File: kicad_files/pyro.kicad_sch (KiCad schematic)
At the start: 14 parts, among them J12 IGN_1, J13 IGN_2, Q1 AO3400A, Q2 AO3400A

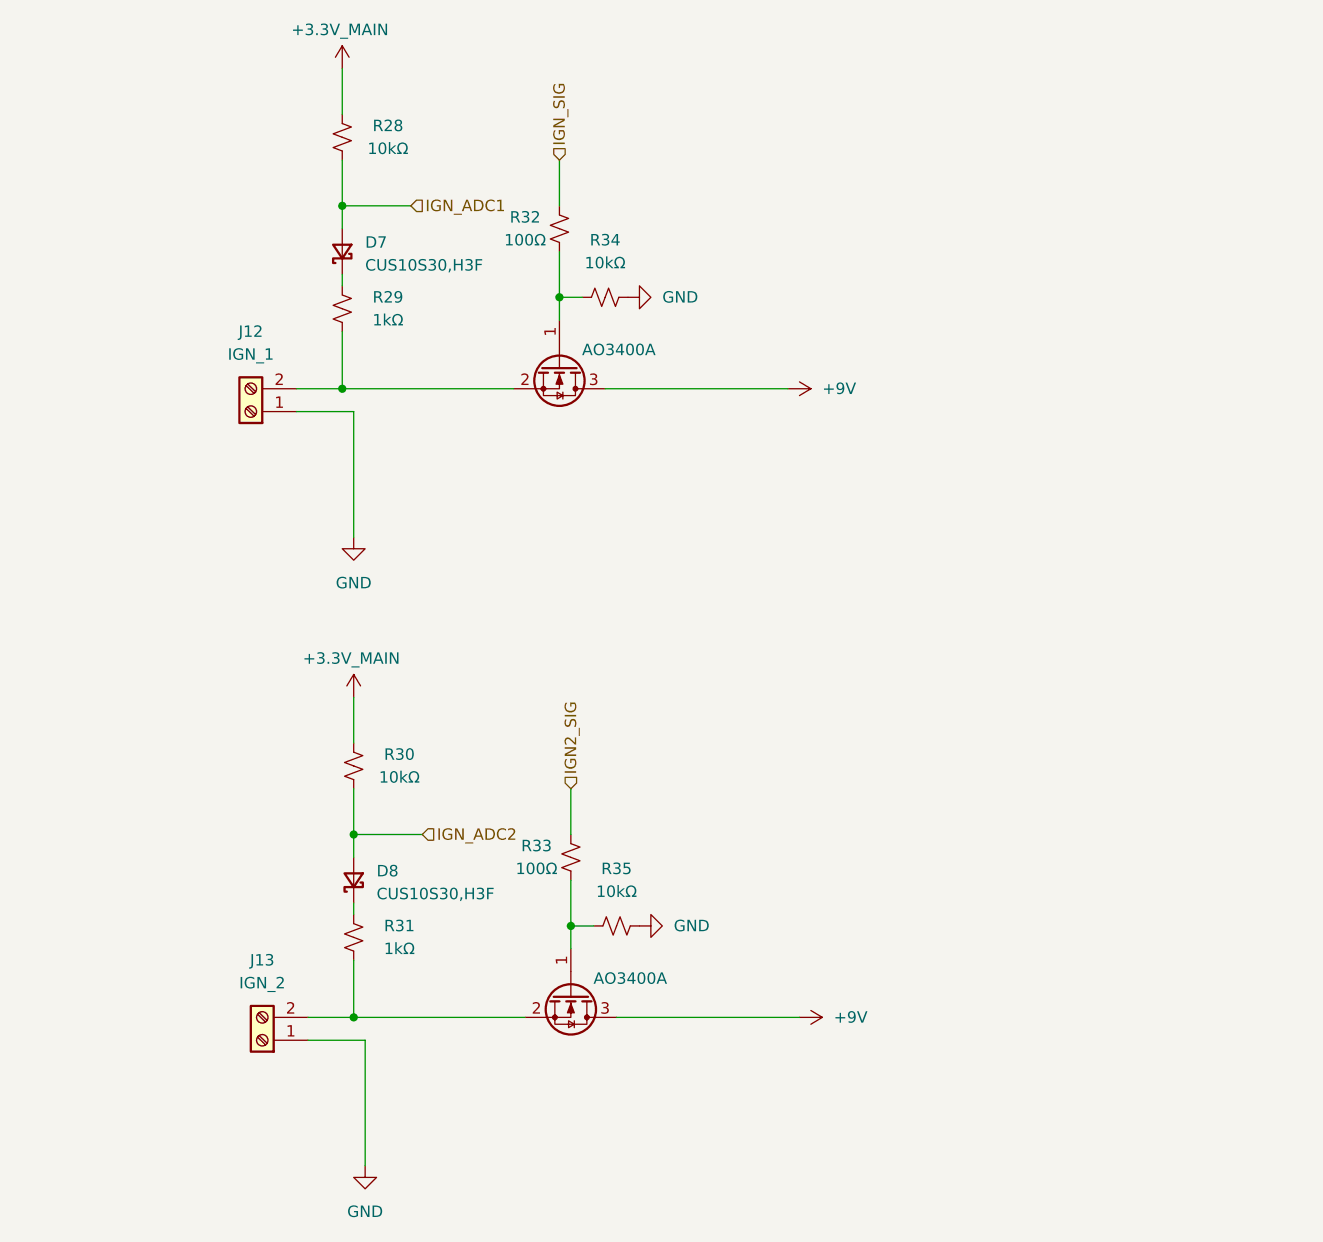
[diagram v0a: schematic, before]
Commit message: fix ign
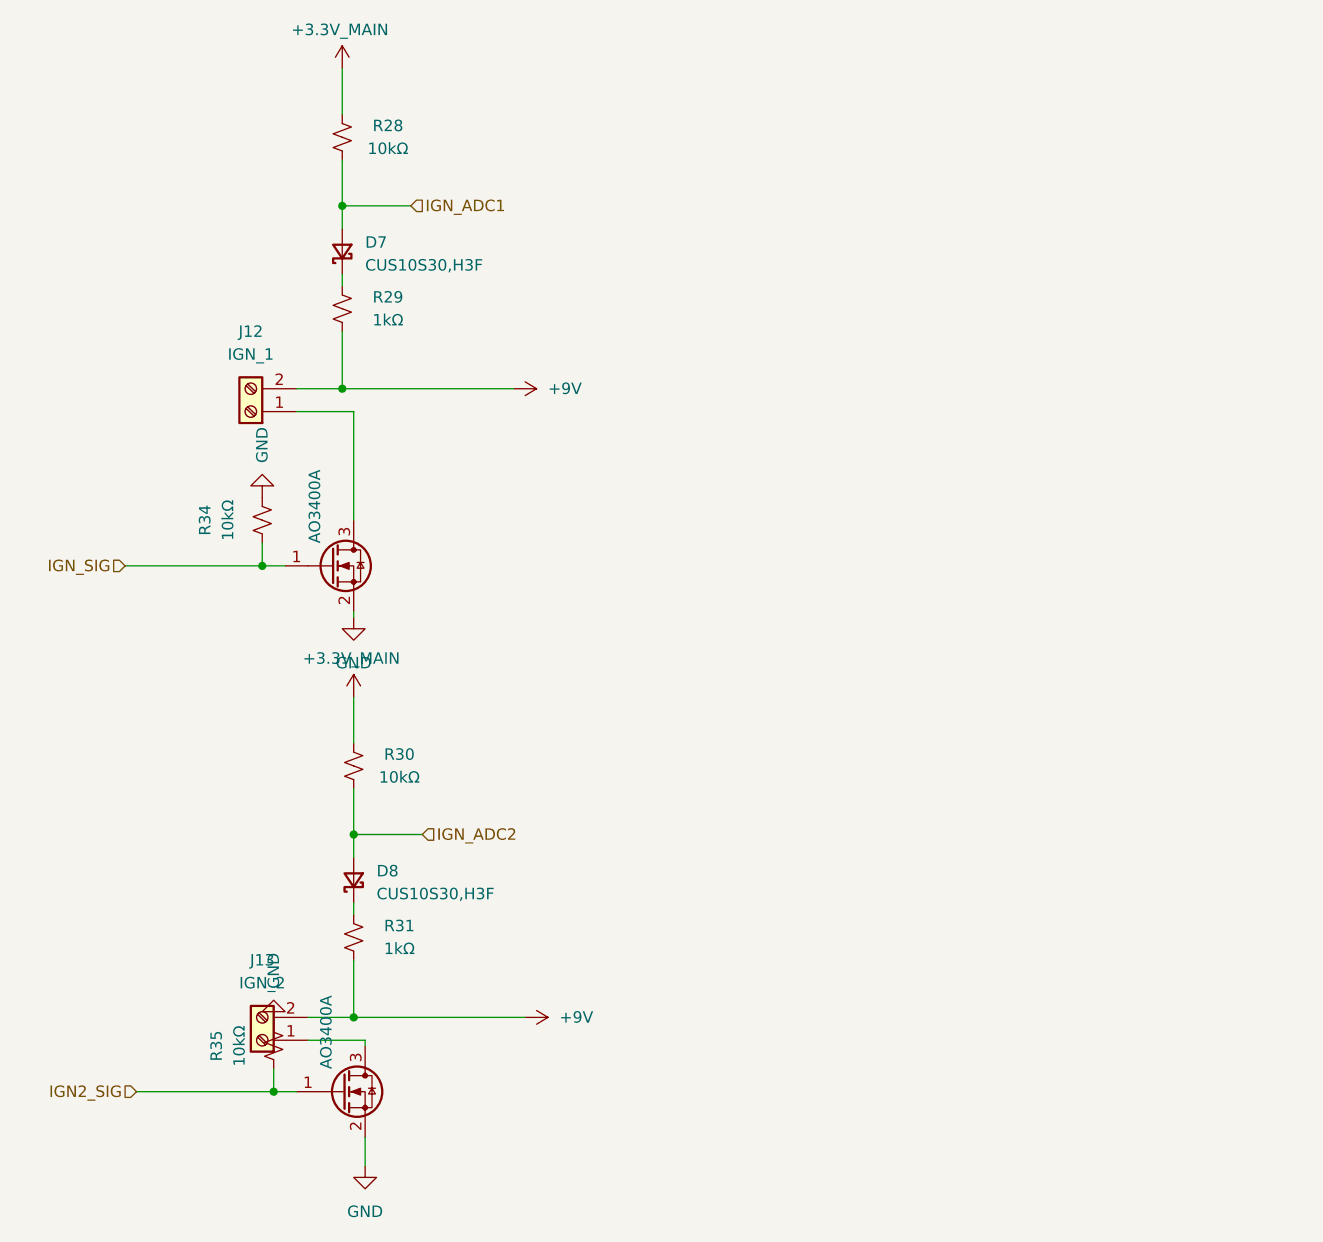
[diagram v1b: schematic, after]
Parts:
- removed R32, R33: 100Ω, Resistor_SMD:R_0603_1608Metric, symbol Device:R_Small_US
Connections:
- net +9V: now also J12.2 (Pin_2), J13.2 (Pin_2), R29.2, R31.2; no longer Q1.3 (D), Q2.3 (D)
- net GND: now also Q1.2 (S), Q2.2 (S); no longer J12.1 (Pin_1), J13.1 (Pin_1)
- net IGN2_SIG: now also Q2.1 (G), R35.1
- net IGN_SIG: now also Q1.1 (G), R34.1
- new net: J13.1 (Pin_1), Q2.3 (D)
- new net: J12.1 (Pin_1), Q1.3 (D)
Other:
- moved on the sheet: R34, R35

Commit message: fix pyro adc
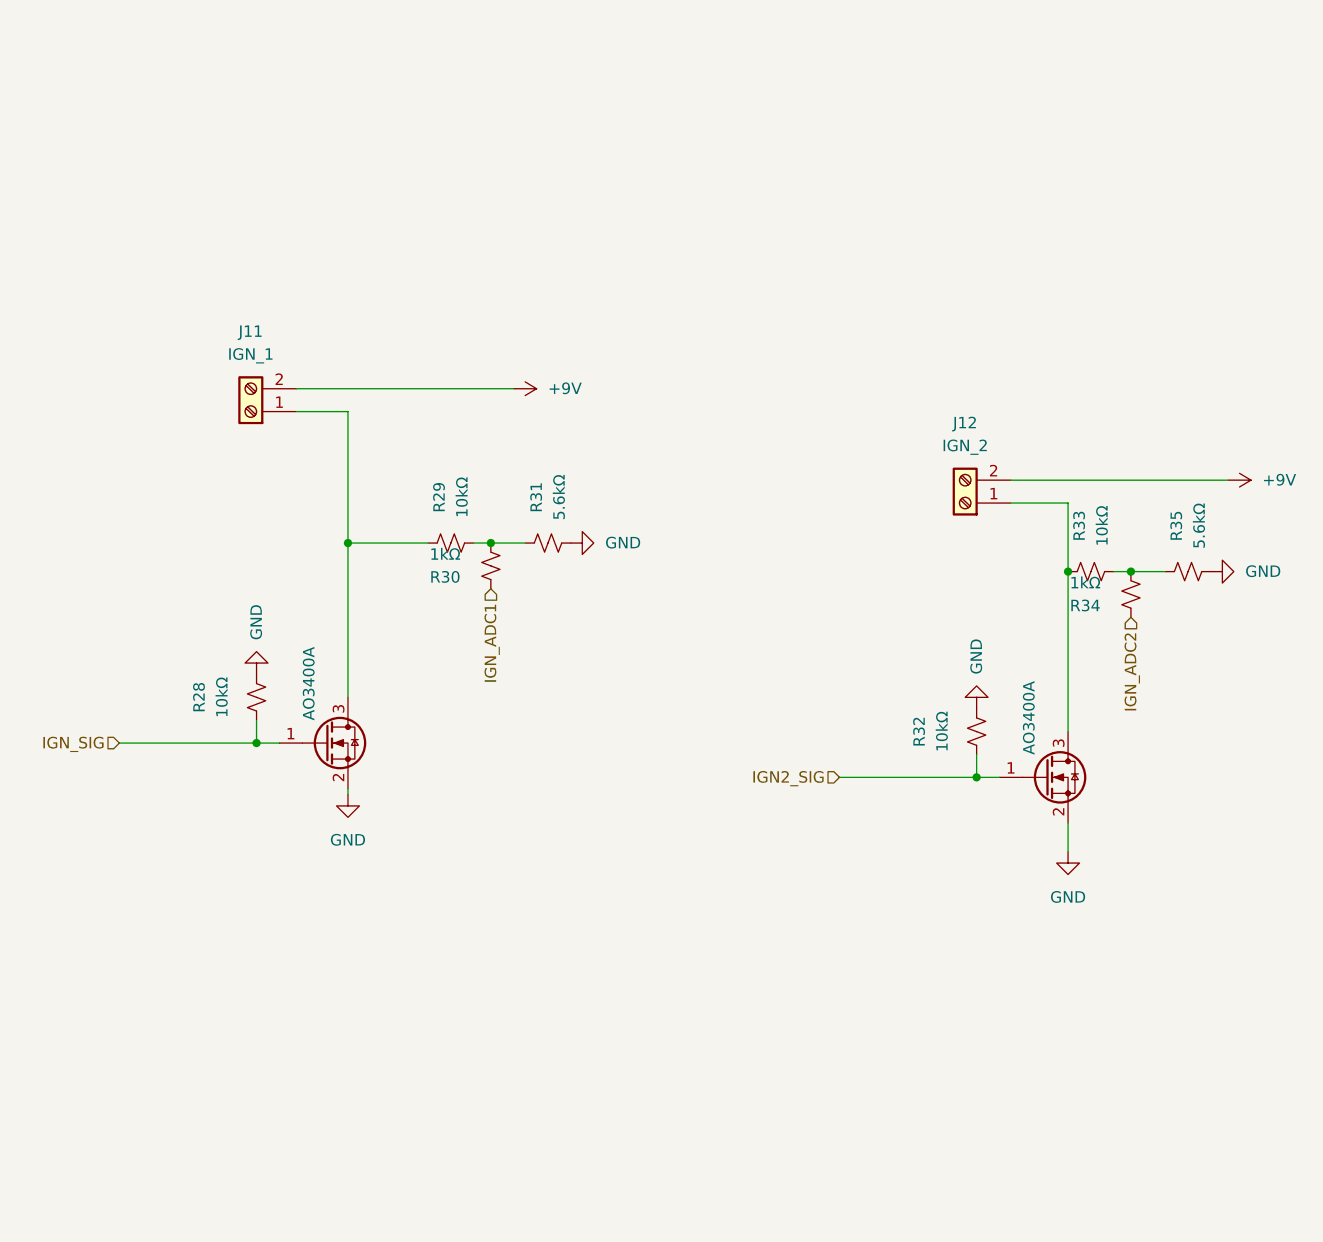
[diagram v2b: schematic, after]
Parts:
- removed D7, D8: CUS10S30,H3F, Diode_SMD:D_SOD-323, symbol Device:D_Schottky_Small
- removed R30: 10kΩ, Resistor_SMD:R_0402_1005Metric, symbol Device:R_Small_US
- added R33: 10kΩ, Resistor_SMD:R_0402_1005Metric, symbol Device:R_Small_US
- added R34: 1kΩ, Resistor_SMD:R_0402_1005Metric, symbol Device:R_Small_US
- added R35: 5.6kΩ, Resistor_SMD:R_0402_1005Metric, symbol Device:R_Small_US
- R30: renamed from R29; footprint Resistor_SMD:R_0805_2012Metric -> Resistor_SMD:R_0402_1005Metric
- R31: value 1kΩ -> 5.6kΩ; footprint Resistor_SMD:R_0805_2012Metric -> Resistor_SMD:R_0402_1005Metric
- renumbered J12 to J11, J13 to J12, R34 to R28, R28 to R29, R35 to R32
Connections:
- net +3.3V_MAIN is gone; now on an unnamed net: R29.1
- net +9V: no longer R30.2, R31.2
- net GND: now also R31.2, R35.2
- net IGN_ADC1: now also R30.1; no longer R29.2
- net IGN_ADC2: now also R34.1
- net at J12.1 (Pin_1), Q2.3 (D): now also R33.1
- net at R31.1: now also R29.2, R30.2
- new net: R33.2, R34.2, R35.1
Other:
- moved on the sheet: J12, R28, R29, R30, R32
